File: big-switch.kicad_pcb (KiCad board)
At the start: 2 copper layers, 76.2 x 76.2 mm, 5 parts, among them J1 Conn_01x07_Socket, SW1 SW_Push, U1 ProMicro

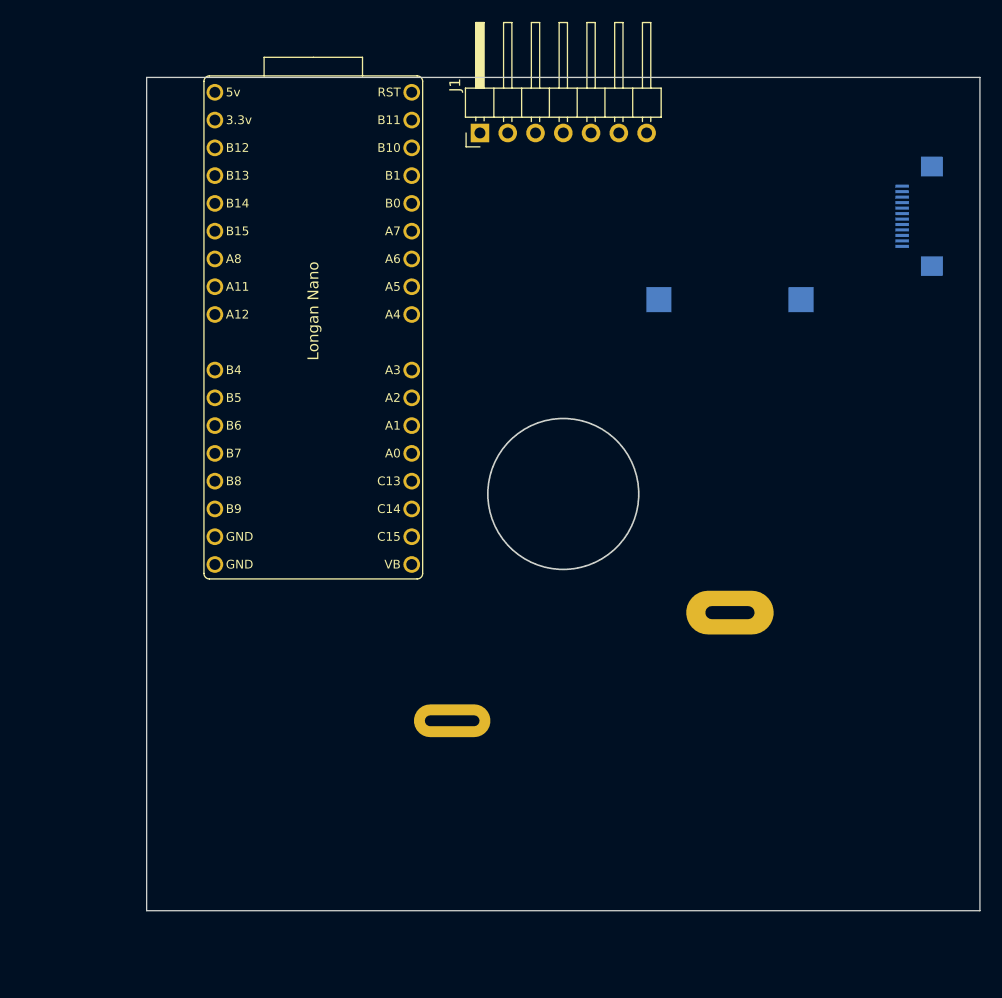
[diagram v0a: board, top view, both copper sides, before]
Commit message: routing ocmplete
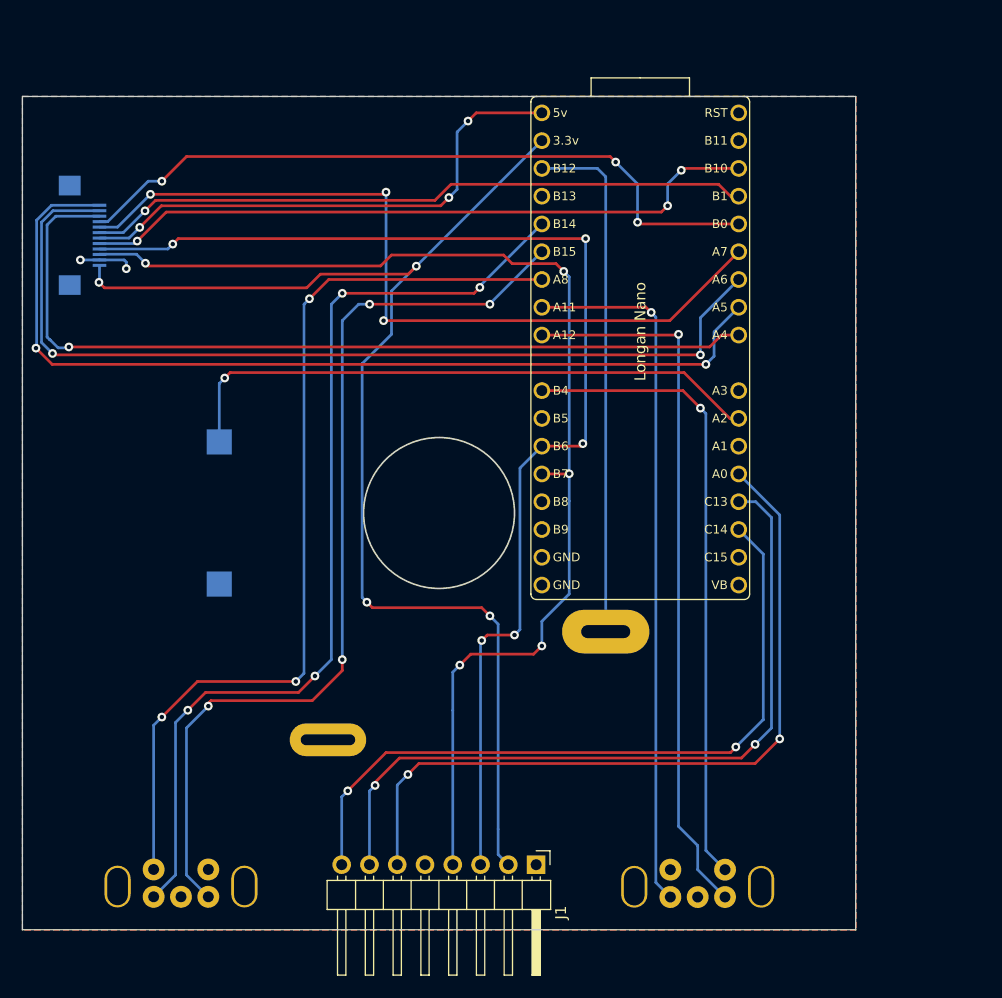
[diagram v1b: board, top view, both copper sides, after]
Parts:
- added SW2: RotaryEncoder_Switch, Keebio-Parts:RotaryEncoder_EC11B-Horizontal-Dual, F.Cu at (89.5, 121.9)
- added SW3: RotaryEncoder_Switch, Keebio-Parts:RotaryEncoder_EC11B-Horizontal-Dual, F.Cu at (136.8, 122.0)
- J1: value Conn_01x07_Socket -> Conn_01x08_Socket; footprint Connector_PinHeader_2.54mm:PinHeader_1x07_P2.54mm_Horizontal -> Connector_PinHeader_2.54mm:PinHeader_1x08_P2.54mm_Horizontal
- U1: value ProMicro -> LonganNano
- moved J2 77.5 mm to (80.0, 62.7), turned to 90 degrees
- moved J1 67.1 mm to (122.0, 120.2), turned to -90 degrees
- moved LS1 50.6 mm to (93.0, 88.1), turned to 90 degrees
- moved U1 30.0 mm to (131.5, 73.0)
- moved SW1 11.5 mm to (113.1, 88.1)
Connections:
- J1 pad 2: VCC -> +3V3
- J1 pad 5: DISP_DC -> unconnected-(J1-Pin_5-Pad5)
- J1 pad 6: DISP_CS -> DISP_DC
- J1 pad 7: DISP_BL -> DISP_CS
- U1 pad 1: unconnected-(U1-TX0/PD3-Pad1) -> +5V
- U1 pad 10: unconnected-(U1-7/PE6-Pad10) -> ENC2_SW
- U1 pad 12: unconnected-(U1-9/PB5-Pad12) -> SCL
- U1 pad 13: unconnected-(U1-10/PB6-Pad13) -> SDA
- U1 pad 16: unconnected-(U1-15/PB1-Pad16) -> GND
- U1 pad 17: unconnected-(U1-A0/PF7-Pad17) -> GND
- U1 pad 2: unconnected-(U1-RX1/PD2-Pad2) -> +3V3
- U1 pad 20: unconnected-(U1-A3/PF4-Pad20) -> DISP_BL
- U1 pad 21: unconnected-(U1-VCC-Pad21) -> DISP_CS
- U1 pad 22: unconnected-(U1-RST-Pad22) -> DISP_DC
- U1 pad 24: unconnected-(U1-RAW-Pad24) -> AUDIO
- U1 pad 25: (no net) -> unconnected-(U1-A3-Pad25)
- U1 pad 26: (no net) -> VIK_CS
- U1 pad 27: (no net) -> SCLK
- U1 pad 28: (no net) -> MISO
- U1 pad 29: (no net) -> MOSI
- U1 pad 3: unconnected-(U1-GND-Pad3) -> SW_1
- U1 pad 30: (no net) -> GPIO_X2
- U1 pad 31: (no net) -> GPIO_X1
- U1 pad 32: (no net) -> VIK_RGB
- U1 pad 33: (no net) -> unconnected-(U1-B11-Pad33)
- U1 pad 34: (no net) -> unconnected-(U1-RST-Pad34)
- U1 pad 5: unconnected-(U1-2/PD1-Pad5) -> ENC1_A
- U1 pad 6: unconnected-(U1-3/PD0-Pad6) -> ENC1_B
- U1 pad 7: unconnected-(U1-4/PD4-Pad7) -> ENC1_SW
- U1 pad 8: unconnected-(U1-5/PC6-Pad8) -> ENC2_A
- U1 pad 9: unconnected-(U1-6/PD7-Pad9) -> ENC2_B
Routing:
- net +3V3: track 0.00 -> 116.0 mm, vias 0 -> 4
- net SCL: track 0.00 -> 109.6 mm, vias 0 -> 5
- net SDA: track 0.00 -> 108.7 mm, vias 0 -> 5
- net ENC1_A: track 0.00 -> 88.3 mm, vias 0 -> 4
- net SCLK: track 0.00 -> 86.5 mm, vias 0 -> 2
- net MISO: track 0.00 -> 85.8 mm, vias 0 -> 2
- net ENC1_B: track 0.00 -> 85.7 mm, vias 0 -> 4
- net ENC1_SW: track 0.00 -> 85.3 mm, vias 0 -> 3
- net VIK_CS: track 0.00 -> 79.5 mm, vias 0 -> 1
- net MOSI: track 0.00 -> 74.5 mm, vias 0 -> 3
- net DISP_DC: track 0.00 -> 69.8 mm, vias 0 -> 2
- net DISP_CS: track 0.00 -> 68.9 mm, vias 0 -> 2
- net DISP_BL: track 0.00 -> 66.0 mm, vias 0 -> 2
- net ENC2_B: track 0.00 -> 65.7 mm, vias 0 -> 1
- net GPIO_X2: track 0.00 -> 65.5 mm, vias 0 -> 3
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- added copper zone on B.Cu, net GND
- added copper zone on F.Cu, net GND
